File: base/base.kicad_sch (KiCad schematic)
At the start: 49 parts, among them J1 24V_PINOUTS_ARM, J10 12V_BUCK_PINOUTS_ARM, J11 12V_BUCK_PINOUTS_ARM, J12 12V_BUCK_PINOUTS_ARM, J14 JETSON_POWER, J15 12V_BUCK_PINOUTS_ARM, J18 BASE_POWER_IN, J19 BuckOut, J2 Conn_01x20_Pin, J20 BatteryIn2, J21 KSMain2, J22 USB_C_Receptacle_USB2.0_14P, J23 MDDPOWER5, J24 MDDPOWER7, J25 MDDPOWER8, J26 MDDPOWER6, J3 BASE_KILL_SWITCH, J4 5VISO_IN, J5 Conn_01x20_Pin, J6 BASE_KILL_SWITCH, J7 12V_BUCK_PINOUTS_ARM, J8 24V_PINOUTS_ARM, J9 12V_BUCK_PINOUTS_ARM, U13 USBLC6-4SC6, U14 USBLC6-4SC6, U15 BNO055, U16 USBLC6-4SC6, U17 USBLC6-4SC6, U18 USBLC6-4SC6

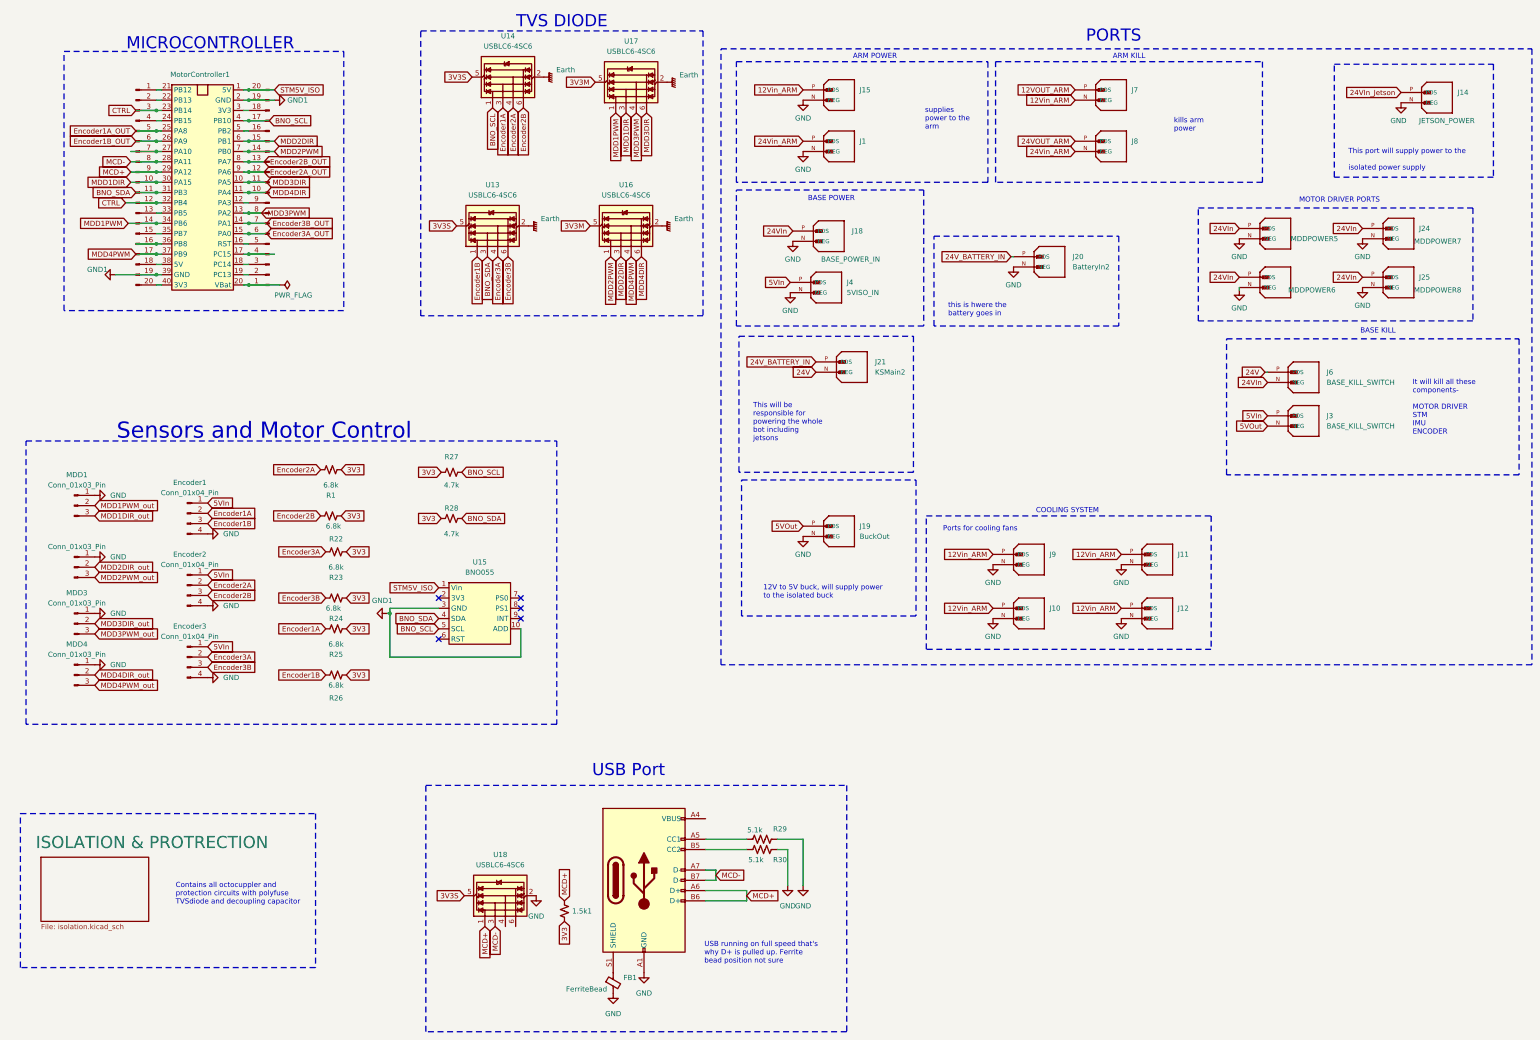
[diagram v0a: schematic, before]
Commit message: fixed labels
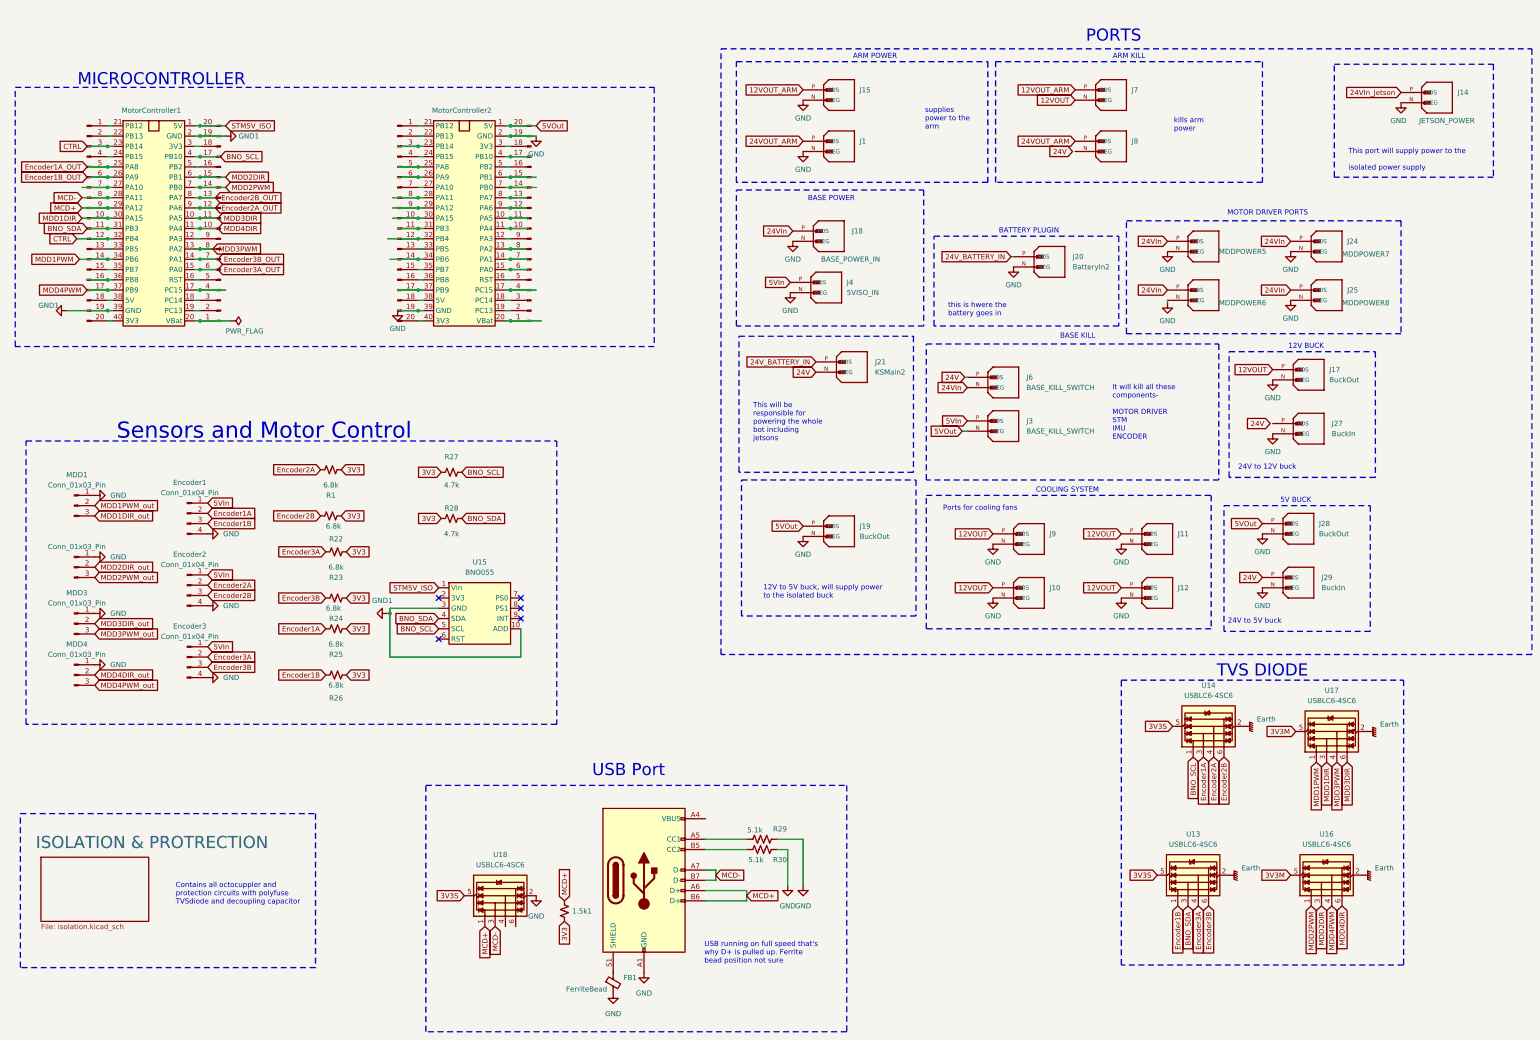
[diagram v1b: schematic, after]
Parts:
- added J13, J16: Conn_01x20_Pin, Connector_PinHeader_2.54mm:PinHeader_1x20_P2.54mm_Vertical, symbol Connector:Conn_01x20_Pin
- added J17, J28: BuckOut, Connector_AMASS:AMASS_XT60PW-M_1x02_P7.20mm_Horizontal, symbol XT60-M:XT60-M
- added J27, J29: BuckIn, Connector_AMASS:AMASS_XT60PW-M_1x02_P7.20mm_Horizontal, symbol XT60-M:XT60-M
- added MotorController2: STM32F411_BP, ROBO:STM32F411-BP, symbol RM_Footprints:STM32F411-BlackPill
- J22: footprint Connector_AMASS:AMASS_XT60PW-M_1x02_P7.20mm_Horizontal -> Connector_USB:USB_C_Receptacle_GCT_USB4105-xx-A_16P_TopMnt_Horizontal
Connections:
- net 12VOUT_ARM: now also J15.P (POS)
- net 24V: now also J29.P (POS)
- net 24VOUT_ARM: now also J1.P (POS)
- net 5VOut: now also J16.20 (Pin_20), J28.P (POS), MotorController2.1 (5V)
- net GND: now also J13.19 (Pin_19), J16.19 (Pin_19), J17.N (NEG), J27.N (NEG), J28.N (NEG), J29.N (NEG), MotorController2.2 (GND), MotorController2.39 (GND)
- net 12Vin_ARM renamed 12VOUT
- net 12VOUT: now also J17.P (POS); no longer J15.P (POS)
- net 24Vin_ARM: no longer names the net of J8.N (NEG)
- net 24Vin_ARM: no longer J1.P (POS)
- new net: J13.1 (Pin_1), MotorController2.21 (PB12)
- new net: J13.10 (Pin_10), MotorController2.30 (PA15)
- new net: J13.11 (Pin_11), MotorController2.31 (PB3)
- new net: J13.12 (Pin_12), MotorController2.32 (PB4)
- new net: J13.13 (Pin_13), MotorController2.33 (PB5)
- new net: J13.14 (Pin_14), MotorController2.34 (PB6)
- new net: J13.15 (Pin_15), MotorController2.35 (PB7)
- new net: J13.16 (Pin_16), MotorController2.36 (PB8)
- new net: J13.17 (Pin_17), MotorController2.37 (PB9)
- new net: J13.18 (Pin_18), MotorController2.38 (5V)
- new net: J13.2 (Pin_2), MotorController2.22 (PB13)
- new net: J13.20 (Pin_20), MotorController2.40 (3V3)
- new net: J13.3 (Pin_3), MotorController2.23 (PB14)
- new net: J13.4 (Pin_4), MotorController2.24 (PB15)
- new net: J13.5 (Pin_5), MotorController2.25 (PA8)
- new net: J13.6 (Pin_6), MotorController2.26 (PA9)
- new net: J13.7 (Pin_7), MotorController2.27 (PA10)
- new net: J13.8 (Pin_8), MotorController2.28 (PA11)
- new net: J13.9 (Pin_9), MotorController2.29 (PA12)
- new net: J16.1 (Pin_1), MotorController2.20 (VBat)
- new net: J16.10 (Pin_10), MotorController2.11 (PA4)
- new net: J16.11 (Pin_11), MotorController2.10 (PA5)
- new net: J16.12 (Pin_12), MotorController2.9 (PA6)
- new net: J16.13 (Pin_13), MotorController2.8 (PA7)
- new net: J16.14 (Pin_14), MotorController2.7 (PB0)
- new net: J16.15 (Pin_15), MotorController2.6 (PB1)
- new net: J16.16 (Pin_16), MotorController2.5 (PB2)
- new net: J16.17 (Pin_17), MotorController2.4 (PB10)
- new net: J16.18 (Pin_18), MotorController2.3 (3V3)
- new net: J16.2 (Pin_2), MotorController2.19 (PC13)
- new net: J16.3 (Pin_3), MotorController2.18 (PC14)
- new net: J16.4 (Pin_4), MotorController2.17 (PC15)
- new net: J16.5 (Pin_5), MotorController2.16 (RST)
- new net: J16.6 (Pin_6), MotorController2.15 (PA0)
- new net: J16.7 (Pin_7), MotorController2.14 (PA1)
- new net: J16.8 (Pin_8), MotorController2.13 (PA2)
- new net: J16.9 (Pin_9), MotorController2.12 (PA3)
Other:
- note added: "12V BUCK"
- note added: "5V BUCK"
- note added: "BATTERY PLUGIN"
- moved on the sheet: J10, J11, J12, J24, J25, J3, J6, J9, MotorController1, U13, U14, U16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
